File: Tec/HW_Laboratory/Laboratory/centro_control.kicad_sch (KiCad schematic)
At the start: 19 parts, among them J36 SPI, J37 USB, J38 IN, J39 USB_C_Receptacle_USB2.0_16P, SW1 SW_Push, SW2 SW_Push, U17 ESP32-S3-WROOM-1, U24 AMS1117-3.3

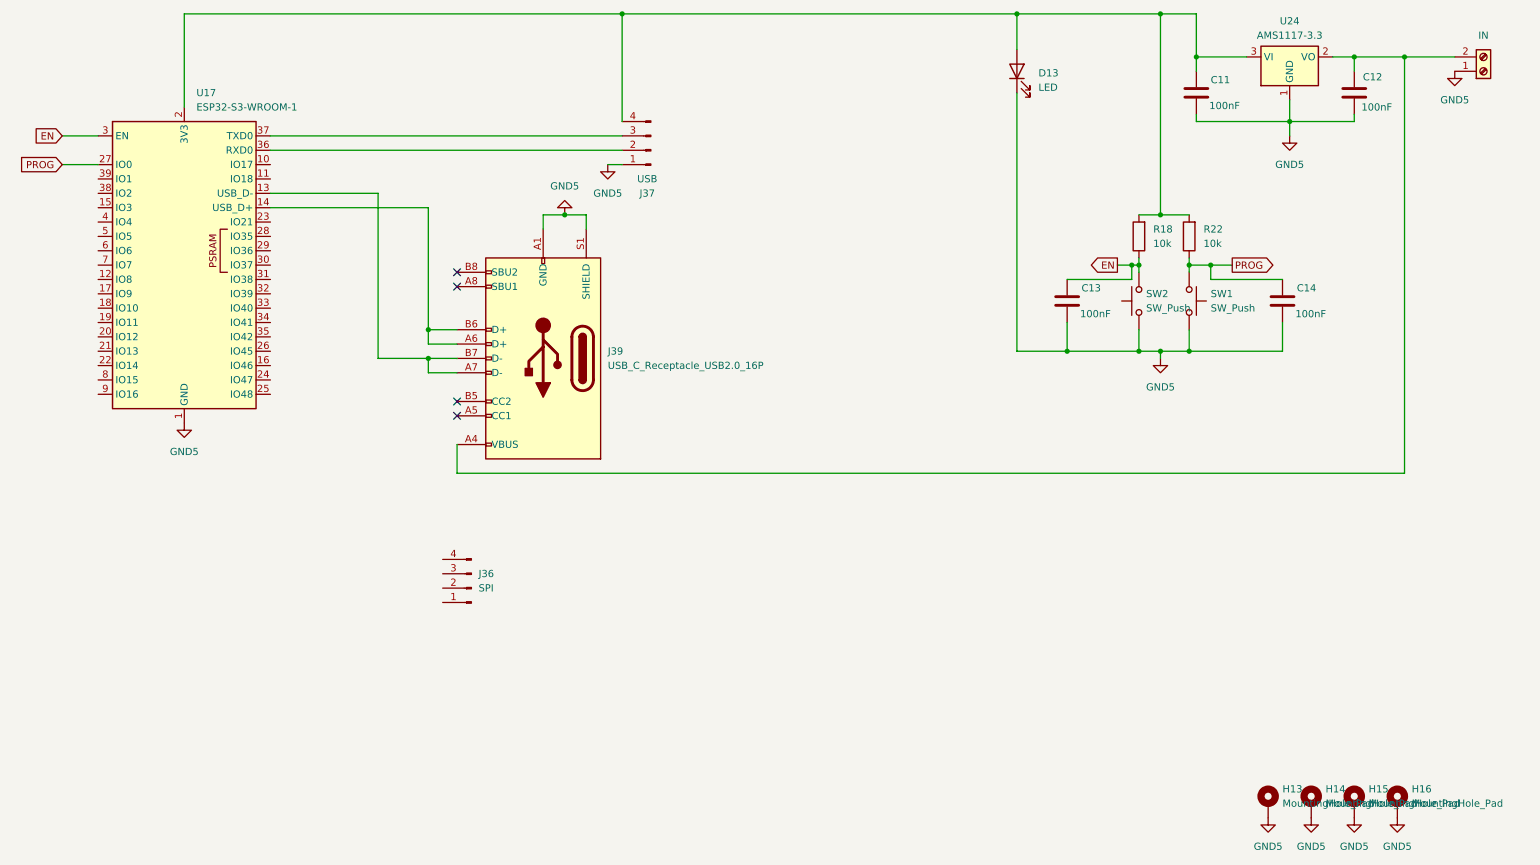
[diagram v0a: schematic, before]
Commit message: Schematics UPDATE
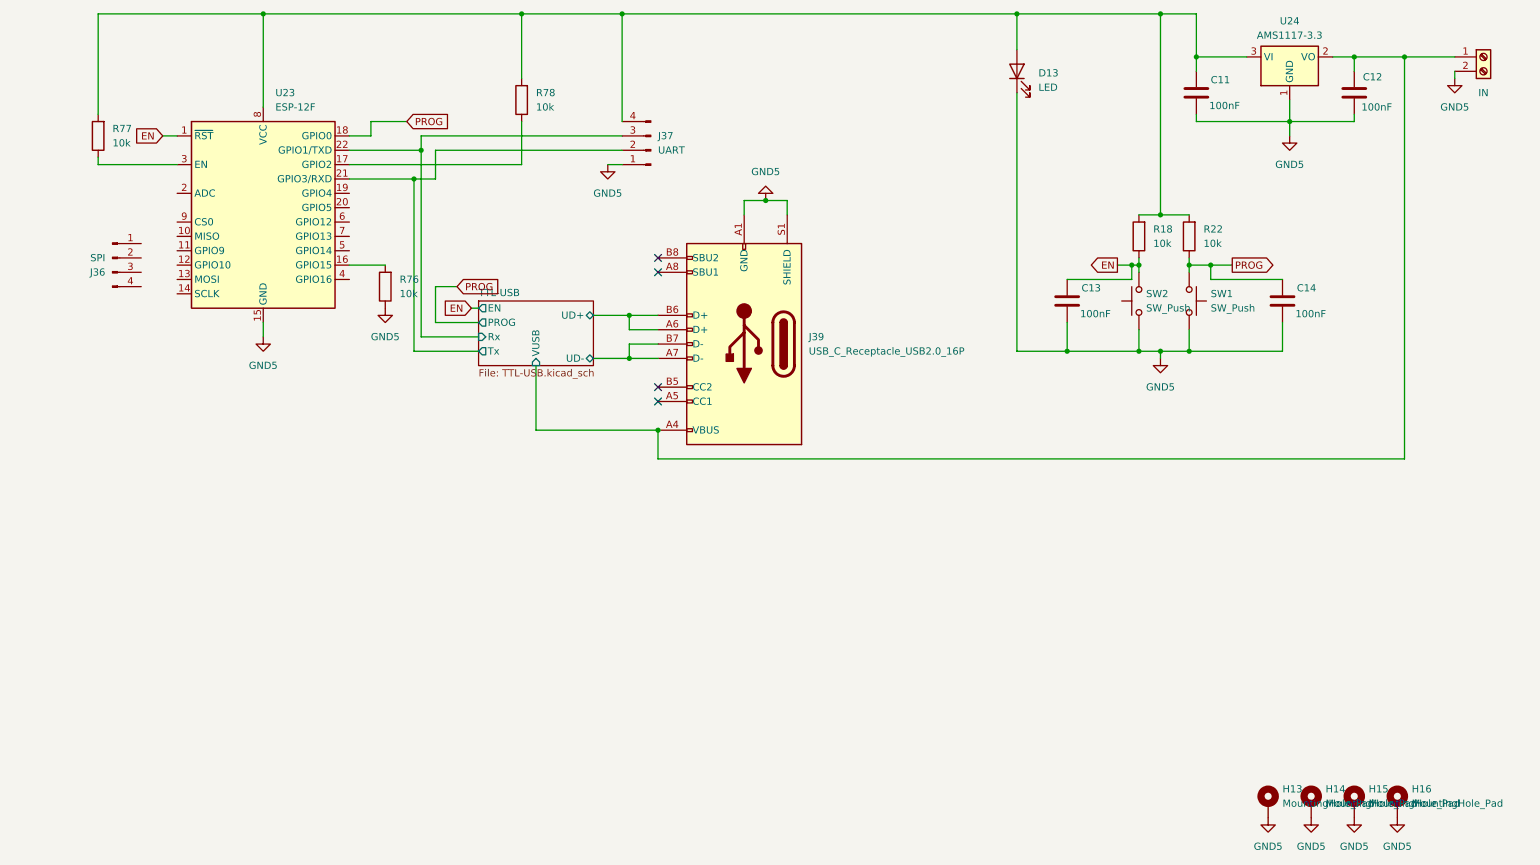
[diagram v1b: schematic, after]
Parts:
- removed U17: ESP32-S3-WROOM-1, RF_Module:ESP32-S3-WROOM-1, symbol RF_Module:ESP32-S3-WROOM-1
- added R76, R77, R78: 10k, Resistor_SMD:R_0603_1608Metric, symbol Device:R
- added U23: ESP-12F, RF_Module:ESP-12E, symbol RF_Module:ESP-12F
- J37: value USB -> UART
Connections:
- net EN: now also U23.1 (~{RST})
- net GND5: now also J38.2 (Pin_2), R76.1, U23.15 (GND); no longer J38.1 (Pin_1)
- net PROG: now also U23.18 (GPIO0)
- net TTL-USB/Tx: now reaches J37.2 (Pin_2)
- net TTL-USB/Tx: now also U23.21 (GPIO3/RXD)
- net TTL-USB/Rx: now reaches J37.3 (Pin_3)
- net TTL-USB/Rx: now also U23.22 (GPIO1/TXD)
- net at C11.1, D13.2 (A), J37.4 (Pin_4)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: now also R77.2, R78.2, U23.8 (VCC)
- net TTL-USB/VUSB: now reaches C12.1, J39.A4 (VBUS), J39.A9 (VBUS), J39.B4 (VBUS), J39.B9 (VBUS), U24.2 (VO)
- net TTL-USB/VUSB: now also J38.1 (Pin_1); no longer J38.2 (Pin_2)
- net TTL-USB/UD+: now reaches J39.A6 (D+), J39.B6 (D+)
- net TTL-USB/UD-: now reaches J39.A7 (D-), J39.B7 (D-)
- new net: R77.1, U23.3 (EN)
- new net: R76.2, U23.16 (GPIO15)
- new net: R78.1, U23.17 (GPIO2)
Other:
- added sheet TTL-USB (TTL-USB.kicad_sch)
- moved on the sheet: J36, J39
